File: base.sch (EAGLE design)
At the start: 24 parts, among them J1 AS0A626-U2SN-7F, SW1 SWS003, U1 XC7A200TFBG676

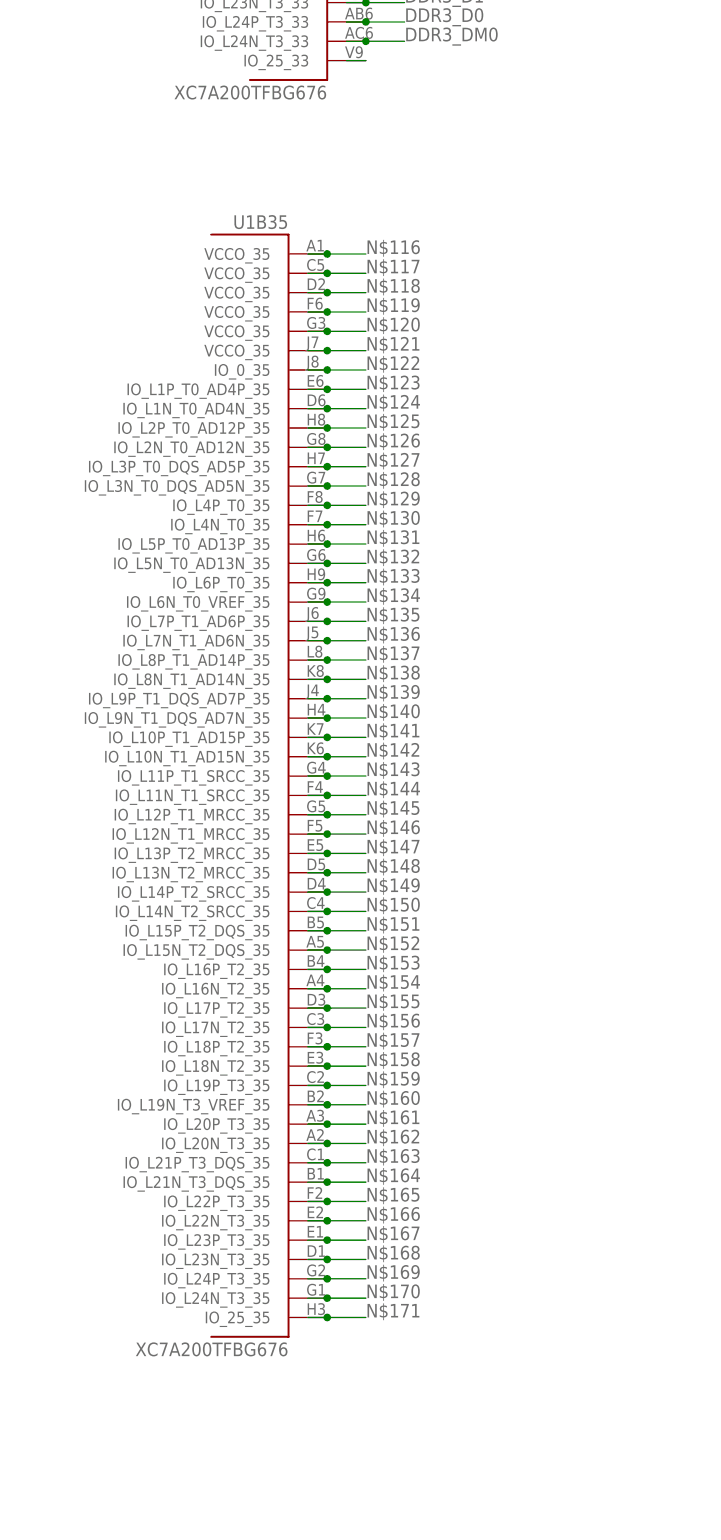
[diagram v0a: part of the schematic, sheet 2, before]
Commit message: adding 35
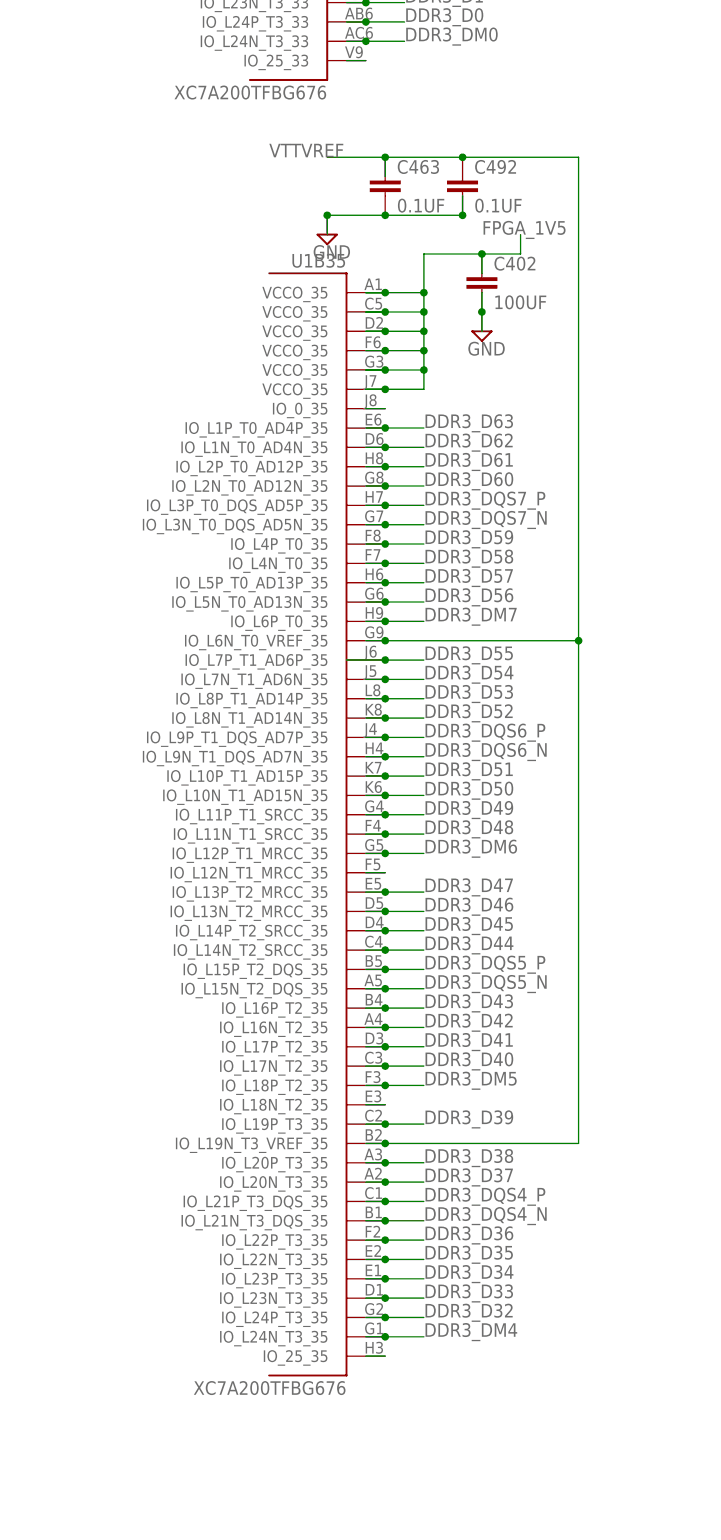
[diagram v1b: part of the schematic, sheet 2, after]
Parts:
- added C402: 100UF, eagle-ltspice:CC1206
- added C463, C492: 0.1UF, eagle-ltspice:CC0402
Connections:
- net N$123 renamed DDR3_D63
- net N$124 renamed DDR3_D62
- net N$125 renamed DDR3_D61
- net N$126 renamed DDR3_D60
- net N$127 renamed DDR3_DQS7_P
- net N$128 renamed DDR3_DQS7_N
- net N$129 renamed DDR3_D59
- net N$130 renamed DDR3_D58
- net N$131 renamed DDR3_D57
- net N$132 renamed DDR3_D56
- net N$133 renamed DDR3_DM7
- net N$135 renamed DDR3_D55
- net N$136 renamed DDR3_D54
- net N$137 renamed DDR3_D53
- net N$138 renamed DDR3_D52
- net N$139 renamed DDR3_DQS6_P
- net N$140 renamed DDR3_DQS6_N
- net N$141 renamed DDR3_D51
- net N$142 renamed DDR3_D50
- net N$143 renamed DDR3_D49
- net N$144 renamed DDR3_D48
- net N$145 renamed DDR3_DM6
- net N$147 renamed DDR3_D47
- net N$148 renamed DDR3_D46
- net N$149 renamed DDR3_D45
- net N$150 renamed DDR3_D44
- net N$151 renamed DDR3_DQS5_P
- net N$152 renamed DDR3_DQS5_N
- net N$153 renamed DDR3_D43
- net N$154 renamed DDR3_D42
- net N$155 renamed DDR3_D41
- net N$156 renamed DDR3_D40
- net N$157 renamed DDR3_DM5
- net N$159 renamed DDR3_D39
- net N$161 renamed DDR3_D38
- net N$162 renamed DDR3_D37
- net N$163 renamed DDR3_DQS4_P
- net N$164 renamed DDR3_DQS4_N
- net N$165 renamed DDR3_D36
- net N$166 renamed DDR3_D35
- net N$167 renamed DDR3_D34
- net N$168 renamed DDR3_D33
- net N$169 renamed DDR3_D32
- net N$170 renamed DDR3_DM4
- removed net N$119: U1B35.VCCO_35@3
- removed net N$134: U1B35.IO_L6N_T0_VREF_35
- removed net N$160: U1B35.IO_L19N_T3_VREF_35
- net FPGA_1V5: now also C402.1, U1B35.VCCO_35@3
- net GND: now also C402.2, C463.2, C492.2
- net VTTVREF: now also C463.1, C492.1, U1B35.IO_L19N_T3_VREF_35, U1B35.IO_L6N_T0_VREF_35
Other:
- moved on the sheet: U1B35
